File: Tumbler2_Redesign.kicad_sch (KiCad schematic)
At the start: 74 parts, among them J1 Conn_01x04, J2 Conn_01x06, J3 USB_C_Receptacle_USB2.0_16P, J4 USB_C_Receptacle_USB2.0_16P, J5 Conn_01x06, Q1 BC817, Q2 BC817, SW1 SW_Push, SW2 SW_Push, SW3 SW_Push, U1 AP63203WU, U2 ESP32-S3-WROOM-1, U3 CP2102N-A02-GQFN28R, U4 AP63205WU, U5 MPU-9250, U6 TB6612FNG, U7 USBLC6-2SC6, U8 USBLC6-2SC6

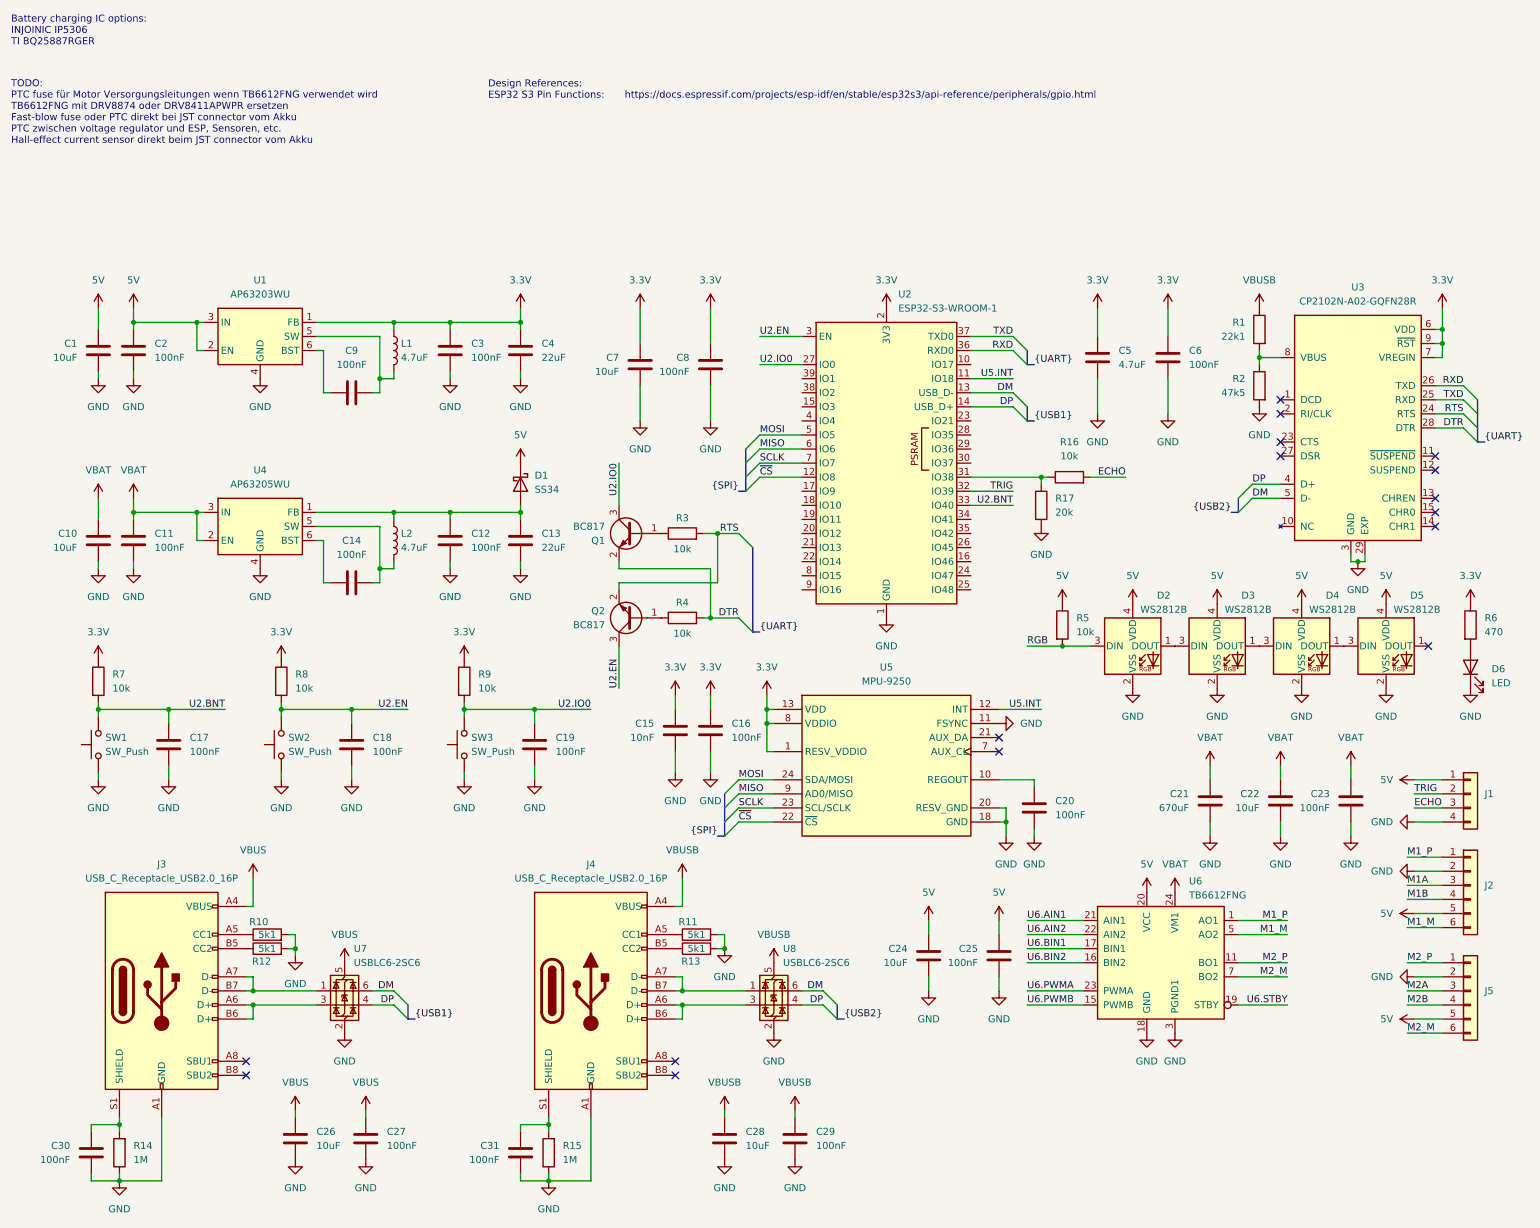
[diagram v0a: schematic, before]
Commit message: Move to hierarchical design
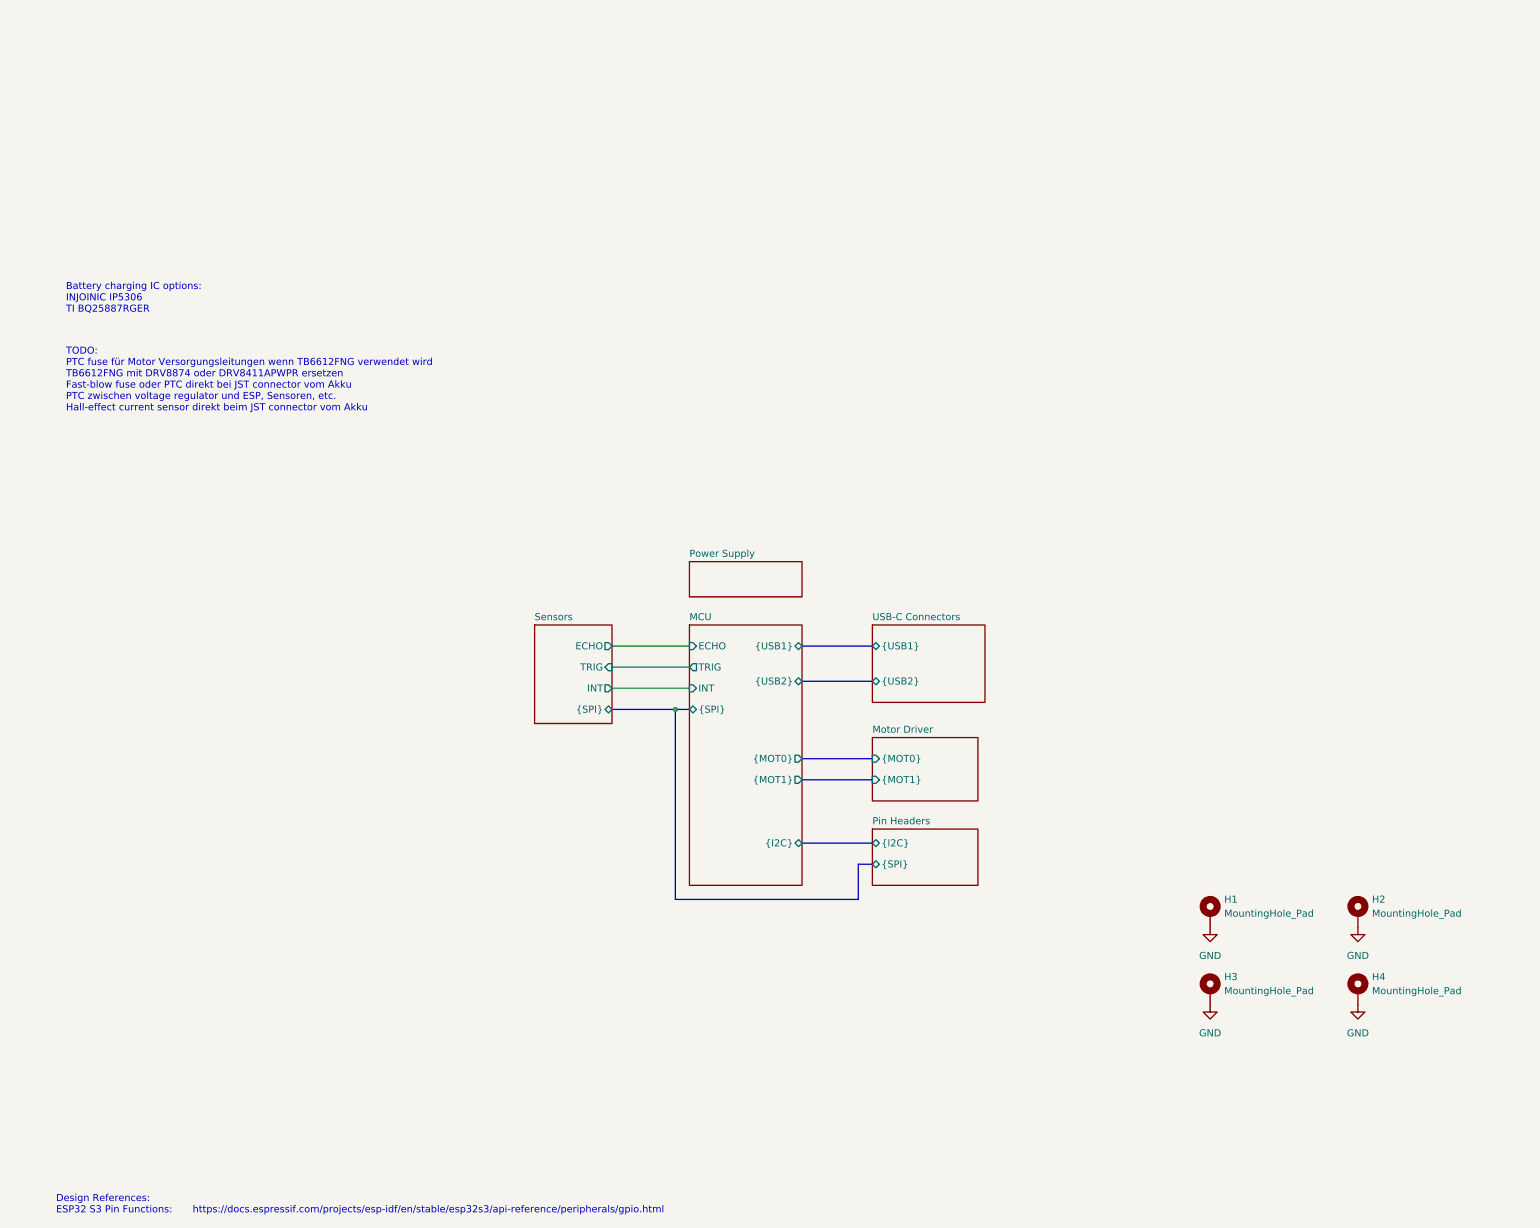
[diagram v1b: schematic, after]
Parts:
- removed C1, C10, C22, C24, C26, C28, C7: 10uF, symbol Device:C
- removed C11, C12, C14, C16, C17, C18, C19, C2, C20, C23, C25, C27, C29, C3, C30, C31, C6, C8, C9: 100nF, symbol Device:C
- removed C13, C4: 22uF, symbol Device:C
- removed C15: 10nF, symbol Device:C
- removed C21: 670uF, symbol Device:C
- removed C5: 4.7uF, symbol Device:C
- removed D1: SS34, Diode_SMD:D_SMA, symbol Diode:SS34
- removed D2, D3, D4, D5: WS2812B, LED_SMD:LED_WS2812B-2020_PLCC4_2.0x2.0mm, symbol LED:WS2812B-2020
- removed D6: LED, symbol Device:LED
- removed J1: Conn_01x04, symbol Connector_Generic:Conn_01x04
- removed J2, J5: Conn_01x06, symbol Connector_Generic:Conn_01x06
- removed J3, J4: USB_C_Receptacle_USB2.0_16P, symbol Connector:USB_C_Receptacle_USB2.0_16P
- removed L1, L2: 4.7uF, symbol Device:L
- removed Q1, Q2: BC817, Package_TO_SOT_SMD:SOT-23, symbol Transistor_BJT:BC817
- removed R1: 22k1, symbol Device:R
- removed R10, R11, R12, R13: 5k1, symbol Device:R
- removed R14, R15: 1M, symbol Device:R
- removed R16, R3, R4, R5, R7, R8, R9: 10k, symbol Device:R
- removed R17: 20k, symbol Device:R
- removed R2: 47k5, symbol Device:R
- removed R6: 470, symbol Device:R
- removed SW1, SW2, SW3: SW_Push, symbol Switch:SW_Push
- removed U1: AP63203WU, Package_TO_SOT_SMD:TSOT-23-6, symbol Regulator_Switching:AP63203WU
- removed U2: ESP32-S3-WROOM-1, RF_Module:ESP32-S3-WROOM-1, symbol RF_Module:ESP32-S3-WROOM-1
- removed U3: CP2102N-A02-GQFN28R, Package_DFN_QFN:QFN-28-1EP_5x5mm_P0.5mm_EP3.35x3.35mm, symbol Tumbler2:CP2102N-A02-GQFN28R
- removed U4: AP63205WU, Package_TO_SOT_SMD:TSOT-23-6, symbol Regulator_Switching:AP63205WU
- removed U5: MPU-9250, Sensor_Motion:InvenSense_QFN-24_3x3mm_P0.4mm, symbol Sensor_Motion:MPU-9250
- removed U6: TB6612FNG, Package_SO:SSOP-24_5.3x8.2mm_P0.65mm, symbol Driver_Motor:TB6612FNG
- removed U7, U8: USBLC6-2SC6, Package_TO_SOT_SMD:SOT-23-6, symbol Power_Protection:USBLC6-2SC6
- added H1, H2, H3, H4: MountingHole_Pad, MountingHole:MountingHole_3mm_Pad, symbol Mechanical:MountingHole_Pad
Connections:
- net GND: now also H1.1, H2.1, H3.1, H4.1
- no-connect marks 16 -> 0
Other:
- added sheet MCU (mcu.kicad_sch)
- added sheet Motor Driver (motor_driver.kicad_sch)
- added sheet Pin Headers (pin_headers.kicad_sch)
- added sheet Power Supply (power_supply.kicad_sch)
- added sheet Sensors (sensors.kicad_sch)
- added sheet USB-C Connectors (usb_c_connector.kicad_sch)
- title: (none) -> Tumbler 2 Redesign
